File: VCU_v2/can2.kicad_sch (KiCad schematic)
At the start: 6 parts, among them U12 MCP2562FD-E/SN

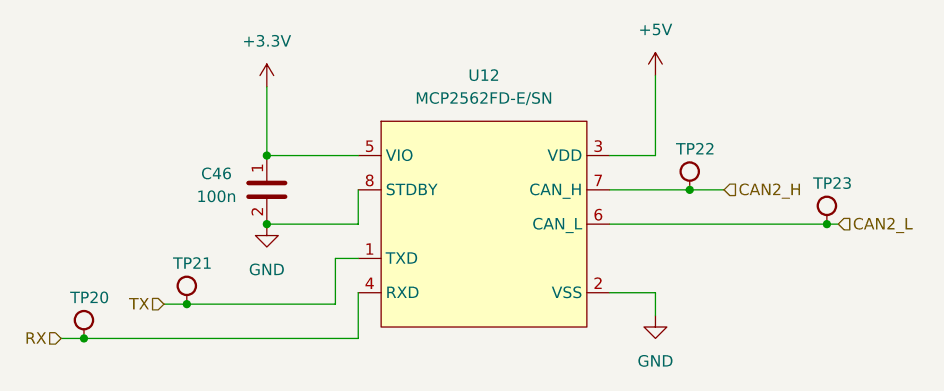
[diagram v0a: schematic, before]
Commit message: vcu v2 schematics done
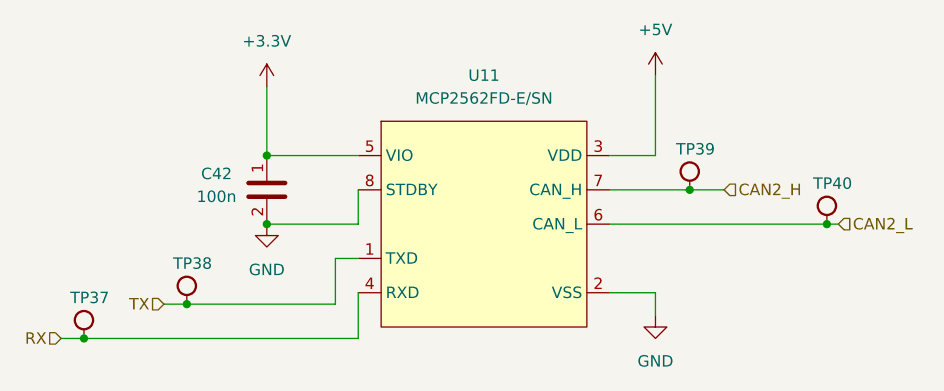
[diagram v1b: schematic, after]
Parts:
- renumbered C46 to C42, TP20 to TP37, TP21 to TP38, TP22 to TP39, TP23 to TP40, U12 to U11
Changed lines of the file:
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@@
 		(dnp no)
 		(fields_autoplaced yes)
-		(property "Reference" "#PWR080"
+		(property "Reference" "#PWR062"
 			(at 156.21 102.87 0)
 			(effects
@@
 			(project "VCU_v1"
 				(path "/4ee6c2ad-9a1b-4276-b3cf-1cc8dc52967e/9e80ce31-2e03-4996-9ce1-7444f7c213d1/123f4073-58d5-4064-8337-35636c3c5d98"
-					(reference "#PWR080")
+					(reference "#PWR062")
 					(unit 1)
 				)
@@
 		(dnp no)
 		(fields_autoplaced yes)
-		(property "Reference" "U12"
+		(property "Reference" "U11"
 			(at 137.16 69.85 0)
 			(effects
@@
 			(project "VCU_v1"
 				(path "/4ee6c2ad-9a1b-4276-b3cf-1cc8dc52967e/9e80ce31-2e03-4996-9ce1-7444f7c213d1/123f4073-58d5-4064-8337-35636c3c5d98"
-					(reference "U12")
+					(reference "U11")
 					(unit 1)
 				)
@@
 		(on_board yes)
 		(dnp no)
-		(property "Reference" "TP23"
+		(property "Reference" "TP40"
 			(at 173.7368 81.1037 0)
 			(effects
@@
 			(project "VCU_v1"
 				(path "/4ee6c2ad-9a1b-4276-b3cf-1cc8dc52967e/9e80ce31-2e03-4996-9ce1-7444f7c213d1/123f4073-58d5-4064-8337-35636c3c5d98"
-					(reference "TP23")
+					(reference "TP40")
 					(unit 1)
 				)
@@
 		(dnp no)
 		(fields_autoplaced yes)
-		(property "Reference" "#PWR079"
+		(property "Reference" "#PWR061"
 			(at 156.21 73.66 0)
 			(effects
@@
 			(project "VCU_v1"
 				(path "/4ee6c2ad-9a1b-4276-b3cf-1cc8dc52967e/9e80ce31-2e03-4996-9ce1-7444f7c213d1/123f4073-58d5-4064-8337-35636c3c5d98"
-					(reference "#PWR079")
+					(reference "#PWR061")
 					(unit 1)
 				)
@@
 		(on_board yes)
 		(dnp no)
-		(property "Reference" "TP20"
+		(property "Reference" "TP37"
 			(at 91.1868 93.8037 0)
 			(effects
@@
 			(project "VCU_v1"
 				(path "/4ee6c2ad-9a1b-4276-b3cf-1cc8dc52967e/9e80ce31-2e03-4996-9ce1-7444f7c213d1/123f4073-58d5-4064-8337-35636c3c5d98"
-					(reference "TP20")
+					(reference "TP37")
 					(unit 1)
 				)
@@
 		(dnp no)
 		(fields_autoplaced yes)
-		(property "Reference" "#PWR078"
+		(property "Reference" "#PWR059"
 			(at 113.03 74.93 0)
 			(effects
@@
 			(project "VCU_v1"
 				(path "/4ee6c2ad-9a1b-4276-b3cf-1cc8dc52967e/9e80ce31-2e03-4996-9ce1-7444f7c213d1/123f4073-58d5-4064-8337-35636c3c5d98"
-					(reference "#PWR078")
+					(reference "#PWR059")
 					(unit 1)
 				)
@@
 		(dnp no)
 		(fields_autoplaced yes)
-		(property "Reference" "#PWR014"
+		(property "Reference" "#PWR060"
 			(at 113.03 92.71 0)
 			(effects
@@
 			(project ""
 				(path "/4ee6c2ad-9a1b-4276-b3cf-1cc8dc52967e/9e80ce31-2e03-4996-9ce1-7444f7c213d1/123f4073-58d5-4064-8337-35636c3c5d98"
-					(reference "#PWR014")
+					(reference "#PWR060")
 					(unit 1)
 				)
@@
 		(on_board yes)
 		(dnp no)
-		(property "Reference" "C46"
+		(property "Reference" "C42"
 			(at 107.442 80.772 0)
 			(effects
@@
 			(project "VCU_v1"
 				(path "/4ee6c2ad-9a1b-4276-b3cf-1cc8dc52967e/9e80ce31-2e03-4996-9ce1-7444f7c213d1/123f4073-58d5-4064-8337-35636c3c5d98"
-					(reference "C46")
+					(reference "C42")
 					(unit 1)
 				)
@@
 		(on_board yes)
 		(dnp no)
-		(property "Reference" "TP22"
+		(property "Reference" "TP39"
 			(at 158.4968 77.2937 0)
 			(effects
@@
 			(project "VCU_v1"
 				(path "/4ee6c2ad-9a1b-4276-b3cf-1cc8dc52967e/9e80ce31-2e03-4996-9ce1-7444f7c213d1/123f4073-58d5-4064-8337-35636c3c5d98"
-					(reference "TP22")
+					(reference "TP39")
 					(unit 1)
 				)
@@
 		(on_board yes)
 		(dnp no)
-		(property "Reference" "TP21"
+		(property "Reference" "TP38"
 			(at 102.6168 89.9937 0)
 			(effects
@@
 			(project "VCU_v1"
 				(path "/4ee6c2ad-9a1b-4276-b3cf-1cc8dc52967e/9e80ce31-2e03-4996-9ce1-7444f7c213d1/123f4073-58d5-4064-8337-35636c3c5d98"
-					(reference "TP21")
+					(reference "TP38")
 					(unit 1)
 				)

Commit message: placements friggin 80% friggin done shoutout epstein
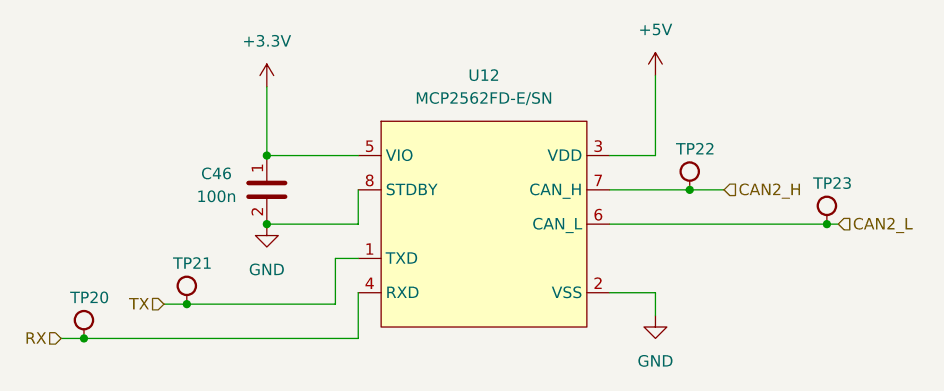
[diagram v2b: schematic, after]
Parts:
- renumbered C42 to C46, TP37 to TP20, TP38 to TP21, TP39 to TP22, TP40 to TP23, U11 to U12
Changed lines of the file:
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@@
 		(dnp no)
 		(fields_autoplaced yes)
-		(property "Reference" "#PWR062"
+		(property "Reference" "#PWR080"
 			(at 156.21 102.87 0)
 			(effects
@@
 			(project "VCU_v1"
 				(path "/4ee6c2ad-9a1b-4276-b3cf-1cc8dc52967e/9e80ce31-2e03-4996-9ce1-7444f7c213d1/123f4073-58d5-4064-8337-35636c3c5d98"
-					(reference "#PWR062")
+					(reference "#PWR080")
 					(unit 1)
 				)
@@
 		(dnp no)
 		(fields_autoplaced yes)
-		(property "Reference" "U11"
+		(property "Reference" "U12"
 			(at 137.16 69.85 0)
 			(effects
@@
 			(project "VCU_v1"
 				(path "/4ee6c2ad-9a1b-4276-b3cf-1cc8dc52967e/9e80ce31-2e03-4996-9ce1-7444f7c213d1/123f4073-58d5-4064-8337-35636c3c5d98"
-					(reference "U11")
+					(reference "U12")
 					(unit 1)
 				)
@@
 		(on_board yes)
 		(dnp no)
-		(property "Reference" "TP40"
+		(property "Reference" "TP23"
 			(at 173.7368 81.1037 0)
 			(effects
@@
 			(project "VCU_v1"
 				(path "/4ee6c2ad-9a1b-4276-b3cf-1cc8dc52967e/9e80ce31-2e03-4996-9ce1-7444f7c213d1/123f4073-58d5-4064-8337-35636c3c5d98"
-					(reference "TP40")
+					(reference "TP23")
 					(unit 1)
 				)
@@
 		(dnp no)
 		(fields_autoplaced yes)
-		(property "Reference" "#PWR061"
+		(property "Reference" "#PWR079"
 			(at 156.21 73.66 0)
 			(effects
@@
 			(project "VCU_v1"
 				(path "/4ee6c2ad-9a1b-4276-b3cf-1cc8dc52967e/9e80ce31-2e03-4996-9ce1-7444f7c213d1/123f4073-58d5-4064-8337-35636c3c5d98"
-					(reference "#PWR061")
+					(reference "#PWR079")
 					(unit 1)
 				)
@@
 		(on_board yes)
 		(dnp no)
-		(property "Reference" "TP37"
+		(property "Reference" "TP20"
 			(at 91.1868 93.8037 0)
 			(effects
@@
 			(project "VCU_v1"
 				(path "/4ee6c2ad-9a1b-4276-b3cf-1cc8dc52967e/9e80ce31-2e03-4996-9ce1-7444f7c213d1/123f4073-58d5-4064-8337-35636c3c5d98"
-					(reference "TP37")
+					(reference "TP20")
 					(unit 1)
 				)
@@
 		(dnp no)
 		(fields_autoplaced yes)
-		(property "Reference" "#PWR059"
+		(property "Reference" "#PWR078"
 			(at 113.03 74.93 0)
 			(effects
@@
 			(project "VCU_v1"
 				(path "/4ee6c2ad-9a1b-4276-b3cf-1cc8dc52967e/9e80ce31-2e03-4996-9ce1-7444f7c213d1/123f4073-58d5-4064-8337-35636c3c5d98"
-					(reference "#PWR059")
+					(reference "#PWR078")
 					(unit 1)
 				)
@@
 		(dnp no)
 		(fields_autoplaced yes)
-		(property "Reference" "#PWR060"
+		(property "Reference" "#PWR014"
 			(at 113.03 92.71 0)
 			(effects
@@
 			(project ""
 				(path "/4ee6c2ad-9a1b-4276-b3cf-1cc8dc52967e/9e80ce31-2e03-4996-9ce1-7444f7c213d1/123f4073-58d5-4064-8337-35636c3c5d98"
-					(reference "#PWR060")
+					(reference "#PWR014")
 					(unit 1)
 				)
@@
 		(on_board yes)
 		(dnp no)
-		(property "Reference" "C42"
+		(property "Reference" "C46"
 			(at 107.442 80.772 0)
 			(effects
@@
 			(project "VCU_v1"
 				(path "/4ee6c2ad-9a1b-4276-b3cf-1cc8dc52967e/9e80ce31-2e03-4996-9ce1-7444f7c213d1/123f4073-58d5-4064-8337-35636c3c5d98"
-					(reference "C42")
+					(reference "C46")
 					(unit 1)
 				)
@@
 		(on_board yes)
 		(dnp no)
-		(property "Reference" "TP39"
+		(property "Reference" "TP22"
 			(at 158.4968 77.2937 0)
 			(effects
@@
 			(project "VCU_v1"
 				(path "/4ee6c2ad-9a1b-4276-b3cf-1cc8dc52967e/9e80ce31-2e03-4996-9ce1-7444f7c213d1/123f4073-58d5-4064-8337-35636c3c5d98"
-					(reference "TP39")
+					(reference "TP22")
 					(unit 1)
 				)
@@
 		(on_board yes)
 		(dnp no)
-		(property "Reference" "TP38"
+		(property "Reference" "TP21"
 			(at 102.6168 89.9937 0)
 			(effects
@@
 			(project "VCU_v1"
 				(path "/4ee6c2ad-9a1b-4276-b3cf-1cc8dc52967e/9e80ce31-2e03-4996-9ce1-7444f7c213d1/123f4073-58d5-4064-8337-35636c3c5d98"
-					(reference "TP38")
+					(reference "TP21")
 					(unit 1)
 				)
